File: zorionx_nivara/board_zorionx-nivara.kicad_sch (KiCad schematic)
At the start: 3 parts, among them U1 ESP32-S3-WROOM-1

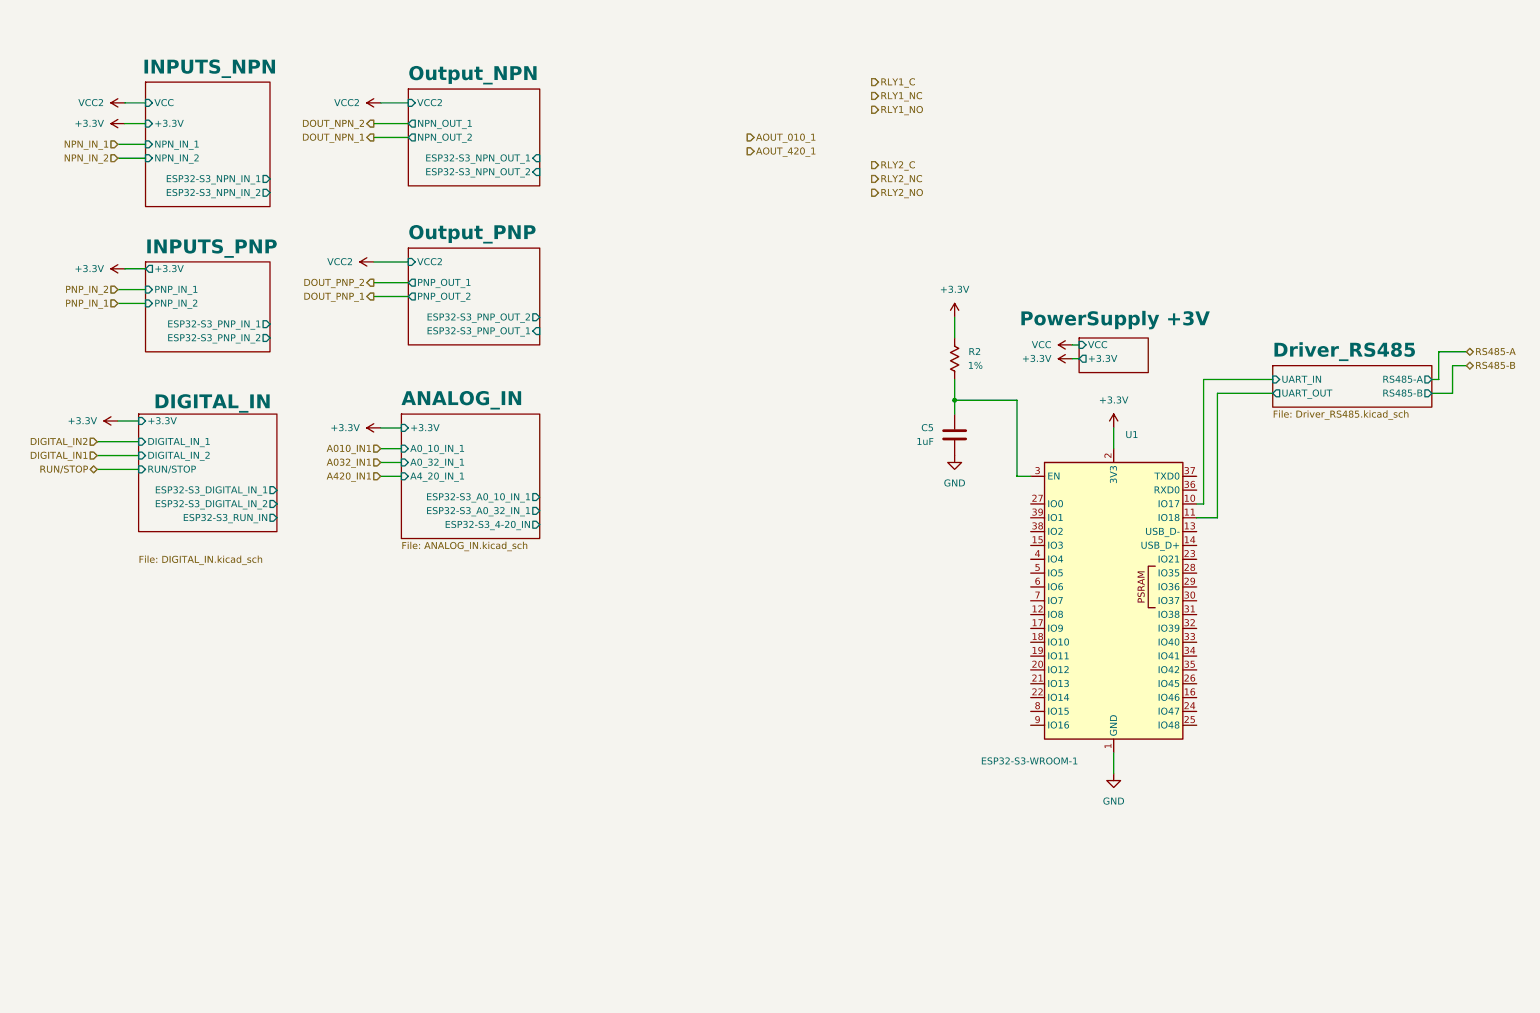
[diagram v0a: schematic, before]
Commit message: Salvado
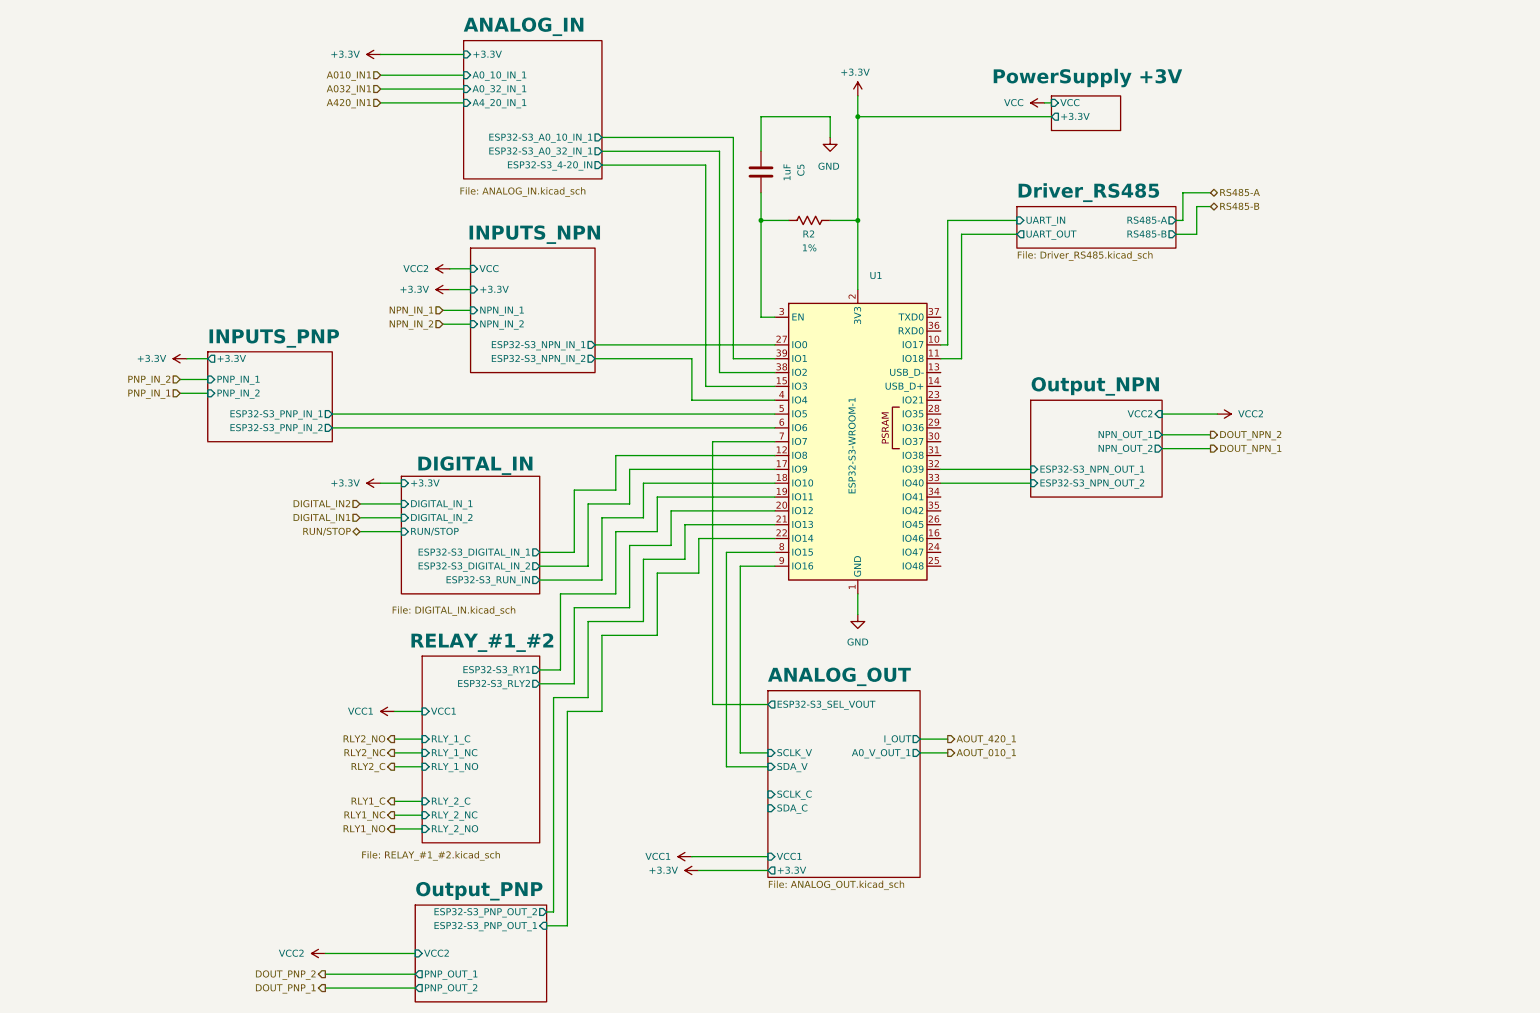
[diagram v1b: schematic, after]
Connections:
- net ANALOG_IN/ESP32-S3_4-20_IN: now also U1.15 (IO3)
- net ANALOG_IN/ESP32-S3_A0_10_IN_1: now also U1.39 (IO1)
- net ANALOG_IN/ESP32-S3_A0_32_IN_1: now also U1.38 (IO2)
- net DIGITAL_IN/ESP32-S3_DIGITAL_IN_1: now also U1.12 (IO8)
- net DIGITAL_IN/ESP32-S3_DIGITAL_IN_2: now also U1.17 (IO9)
- net DIGITAL_IN/ESP32-S3_RUN_IN: now also U1.18 (IO10)
- net INPUTS_NPN/ESP32-S3_NPN_IN_1: now also U1.27 (IO0)
- net INPUTS_NPN/ESP32-S3_NPN_IN_2: now also U1.4 (IO4)
- net INPUTS_PNP/ESP32-S3_PNP_IN_1: now also U1.5 (IO5)
- net INPUTS_PNP/ESP32-S3_PNP_IN_2: now also U1.6 (IO6)
- net Output_NPN/ESP32-S3_NPN_OUT_1: now also U1.32 (IO39)
- net Output_NPN/ESP32-S3_NPN_OUT_2: now also U1.33 (IO40)
- net Output_PNP/ESP32-S3_PNP_OUT_1: now also U1.22 (IO14)
- net Output_PNP/ESP32-S3_PNP_OUT_2: now also U1.21 (IO13)
- net RELAY_#1_#2/ESP32-S3_RY1: now reaches U1.19 (IO11)
- net RELAY_#1_#2/ESP32-S3_RLY2: now reaches U1.20 (IO12)
- net ANALOG_OUT/ESP32-S3_SEL_VOUT: now reaches U1.7 (IO7)
- net ANALOG_OUT/SDA_V: now reaches U1.8 (IO15)
- net ANALOG_OUT/SCLK_V: now reaches U1.9 (IO16)
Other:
- added sheet ANALOG_OUT (ANALOG_OUT.kicad_sch)
- added sheet RELAY_#1_#2 (RELAY_#1_#2.kicad_sch)
- moved on the sheet: C5, R2, U1
